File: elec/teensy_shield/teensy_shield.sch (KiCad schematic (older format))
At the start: 0 parts

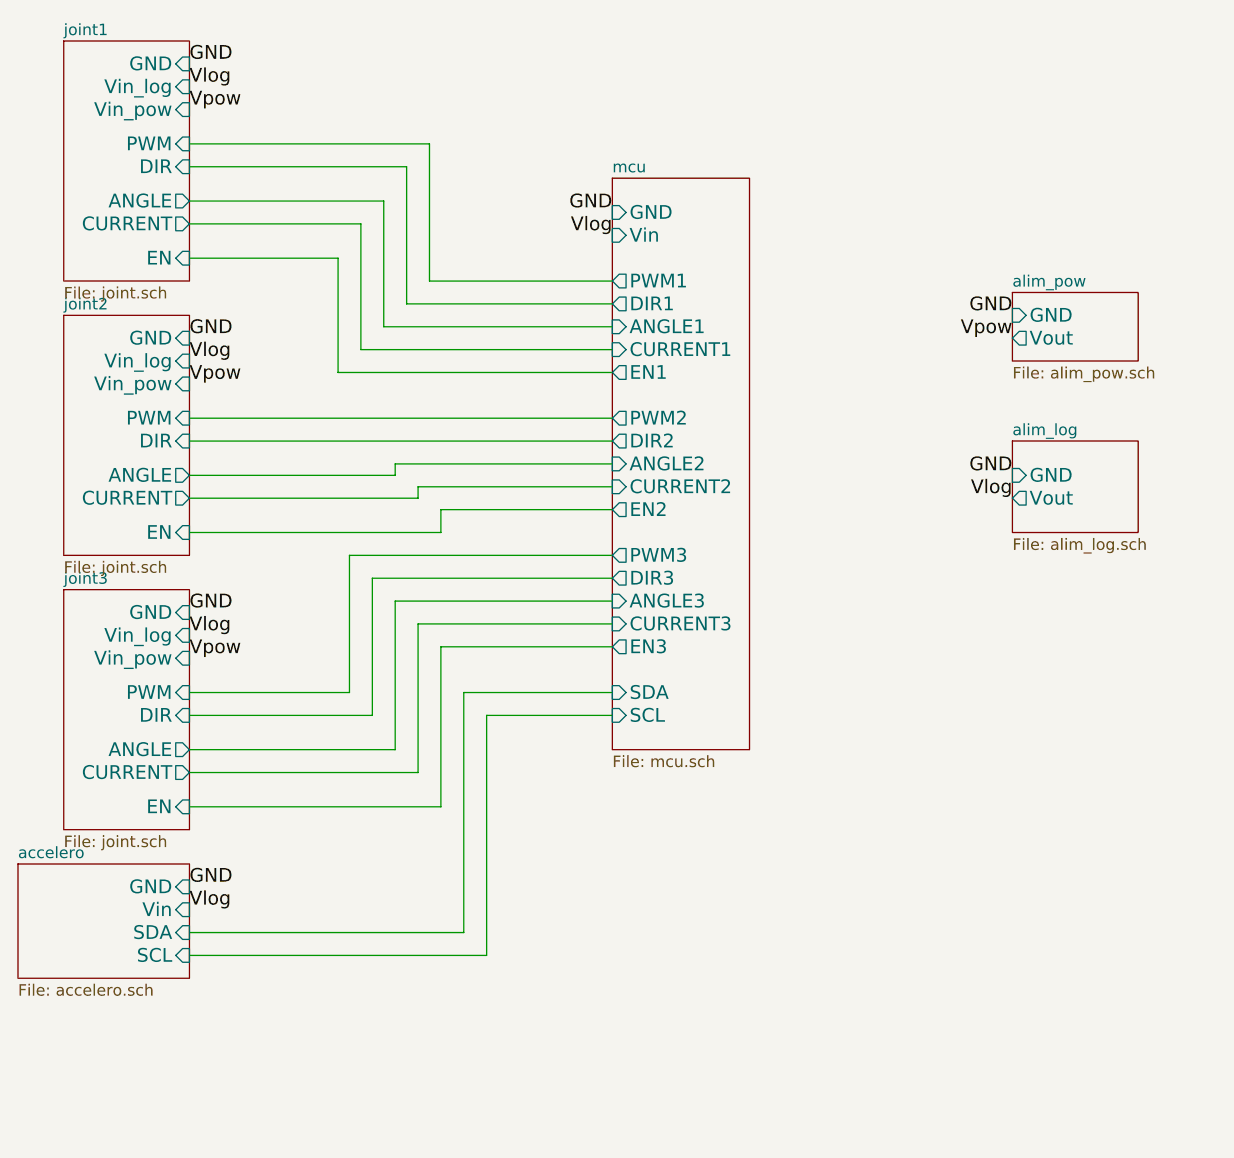
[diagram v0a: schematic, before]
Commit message: Completed new board schematics.
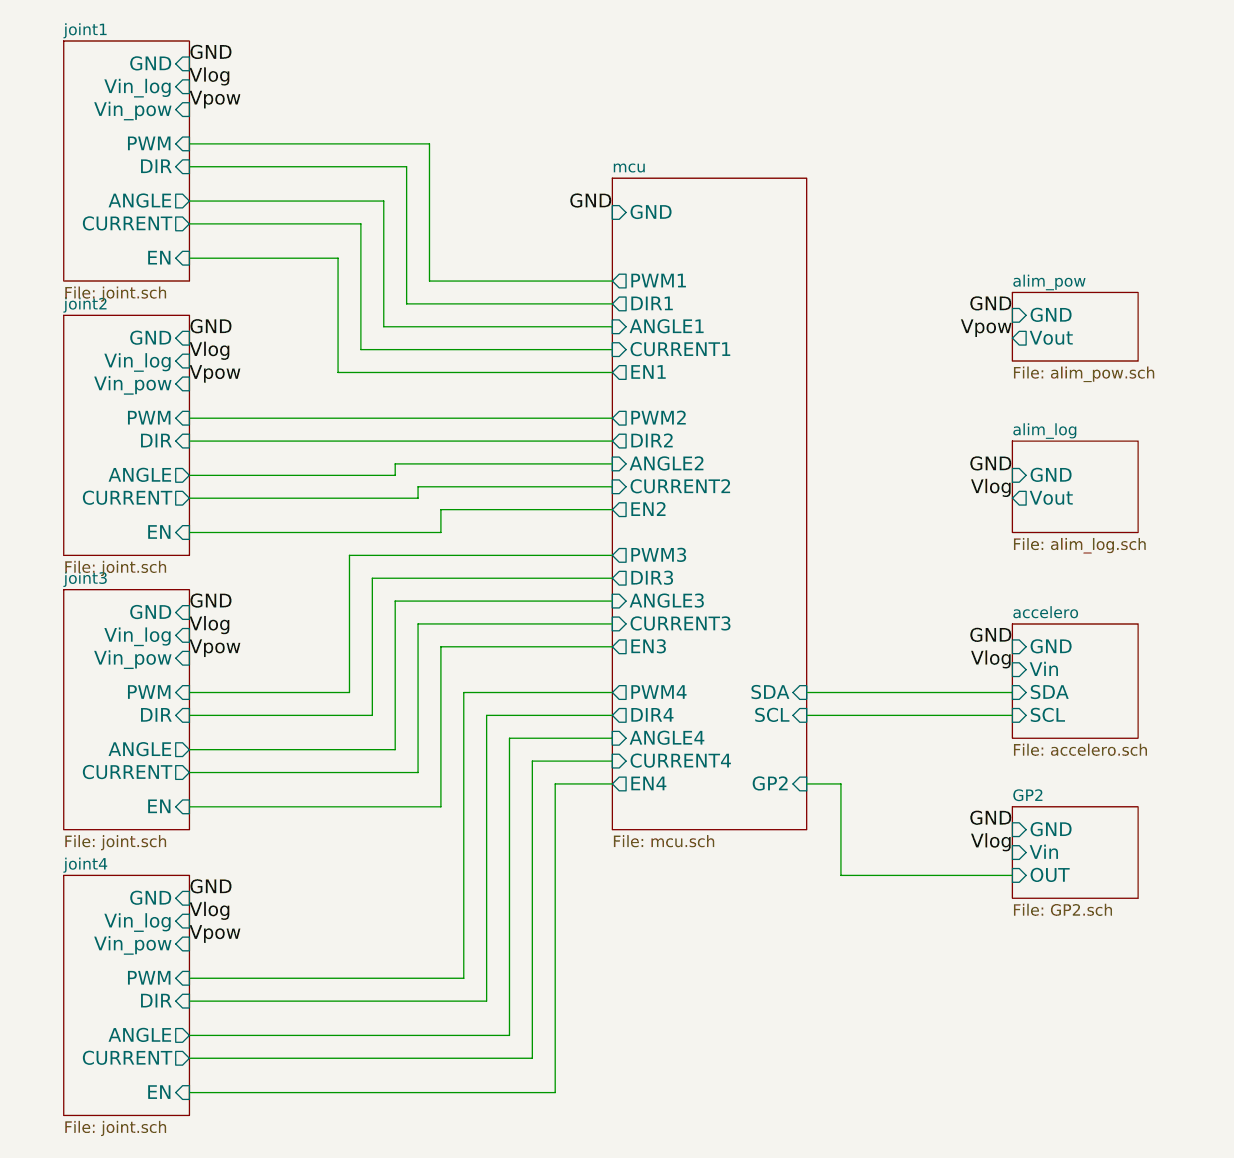
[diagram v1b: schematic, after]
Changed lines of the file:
@@
 LIBS:contrib
 LIBS:valves
+LIBS:arduino_shieldsNCL
+LIBS:teensy
+LIBS:pololu
+LIBS:teensy_shield-cache
 EELAYER 24 0
 EELAYER END
 $Descr A4 11693 8268
 encoding utf-8
-Sheet 1 26
+Sheet 1 34
 Title ""
 Date ""
@@
 $EndDescr
 $Sheet
-S 6300 1550 600  2500
+S 6300 1550 850  2850
 U 55E5CC66
 F0 "mcu" 50
 F1 "mcu.sch" 50
 F2 "GND" I L 6300 1700 60
-F3 "Vin" I L 6300 1800 60
 F4 "PWM1" O L 6300 2000 60
 F5 "DIR1" O L 6300 2100 60
@@
 F17 "CURRENT3" I L 6300 3500 60
 F18 "EN3" O L 6300 3600 60
-F19 "SDA" I L 6300 3800 60
-F20 "SCL" I L 6300 3900 60
-$EndSheet
-$Sheet
-S 3700 4550 750  500
+F19 "SDA" I R 7150 3800 60
+F20 "SCL" I R 7150 3900 60
+F21 "PWM4" O L 6300 3800 60
+F22 "DIR4" O L 6300 3900 60
+F23 "ANGLE4" I L 6300 4000 60
+F24 "CURRENT4" I L 6300 4100 60
+F25 "EN4" O L 6300 4200 60
+F26 "GP2" I R 7150 4200 60
+$EndSheet
+$Sheet
+S 8050 3500 550  500
 U 55E614B3
 F0 "accelero" 50
 F1 "accelero.sch" 50
-F2 "GND" I R 4450 4650 60
-F3 "Vin" I R 4450 4750 60
-F4 "SDA" I R 4450 4850 60
-F5 "SCL" I R 4450 4950 60
+F2 "GND" I L 8050 3600 60
+F3 "Vin" I L 8050 3700 60
+F4 "SDA" I L 8050 3800 60
+F5 "SCL" I L 8050 3900 60
 $EndSheet
 $Sheet
@@
 Wire Wire Line
 	5550 4300 4450 4300
-Wire Wire Line
-	6300 3800 5650 3800
-Wire Wire Line
-	5650 3800 5650 4850
-Wire Wire Line
-	5650 4850 4450 4850
-Wire Wire Line
-	6300 3900 5750 3900
-Wire Wire Line
-	5750 3900 5750 4950
-Wire Wire Line
-	5750 4950 4450 4950
 $Sheet
 S 8050 2050 550  300
@@
 Text Label 4450 3450 0    60   ~ 0
 GND
-Text Label 4450 4650 0    60   ~ 0
+Text Label 8050 3600 2    60   ~ 0
 GND
 Text Label 4450 1150 0    60   ~ 0
@@
 Text Label 4450 3550 0    60   ~ 0
 Vlog
-Text Label 4450 4750 0    60   ~ 0
-Vlog
-Text Label 6300 1800 2    60   ~ 0
+Text Label 8050 3700 2    60   ~ 0
 Vlog
 Text Label 8050 2950 2    60   ~ 0
@@
 Text Label 4450 3650 0    60   ~ 0
 Vpow
+$Sheet
+S 3900 4600 550  1050
+U 55E6307C
+F0 "joint4" 50
+F1 "joint.sch" 50
+F2 "GND" I R 4450 4700 60
+F3 "Vin_log" I R 4450 4800 60
+F4 "Vin_pow" I R 4450 4900 60
+F5 "PWM" I R 4450 5050 60
+F6 "DIR" I R 4450 5150 60
+F7 "ANGLE" O R 4450 5300 60
+F8 "CURRENT" O R 4450 5400 60
+F9 "EN" I R 4450 5550 60
+$EndSheet
+Wire Wire Line
+	4450 5050 5650 5050
+Wire Wire Line
+	5650 5050 5650 3800
+Wire Wire Line
+	5650 3800 6300 3800
+Wire Wire Line
+	4450 5150 5750 5150
+Wire Wire Line
+	5750 5150 5750 3900
+Wire Wire Line
+	5750 3900 6300 3900
+Wire Wire Line
+	4450 5300 5850 5300
+Wire Wire Line
+	5850 5300 5850 4000
+Wire Wire Line
+	5850 4000 6300 4000
+Wire Wire Line
+	4450 5400 5950 5400
+Wire Wire Line
+	5950 5400 5950 4100
+Wire Wire Line
+	5950 4100 6300 4100
+Wire Wire Line
+	4450 5550 6050 5550
+Wire Wire Line
+	6050 5550 6050 4200
+Wire Wire Line
+	6050 4200 6300 4200
+$Sheet
+S 8050 4300 550  400
+U 55E7E869
+F0 "GP2" 50
+F1 "GP2.sch" 50
+F2 "GND" I L 8050 4400 60
+F3 "Vin" I L 8050 4500 60
+F4 "OUT" I L 8050 4600 60
+$EndSheet
+Wire Wire Line
+	8050 4600 7300 4600
+Wire Wire Line
+	7300 4600 7300 4200
+Wire Wire Line
+	7300 4200 7150 4200
+Wire Wire Line
+	8050 3900 7150 3900
+Wire Wire Line
+	8050 3800 7150 3800
+Text Label 4450 4700 0    60   ~ 0
+GND
+Text Label 4450 4800 0    60   ~ 0
+Vlog
+Text Label 4450 4900 0    60   ~ 0
+Vpow
+Text Label 8050 4400 2    60   ~ 0
+GND
+Text Label 8050 4500 2    60   ~ 0
+Vlog
 $EndSCHEMATC
